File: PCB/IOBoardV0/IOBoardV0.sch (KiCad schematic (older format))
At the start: 28 parts, among them J2 RJ45_2, J3 RJ45_2, J4 RJ45_2, J5 RJ45_2, J6 RJ45_2, J7 RJ45_2, J8 RJ45_2, J9 RJ45_2, P1 RASPBERRY_HAT, U1 74LS04, U2 74LS138, U3 74LS164, U4 74LS373, U5 74LS74, U6 74LS165

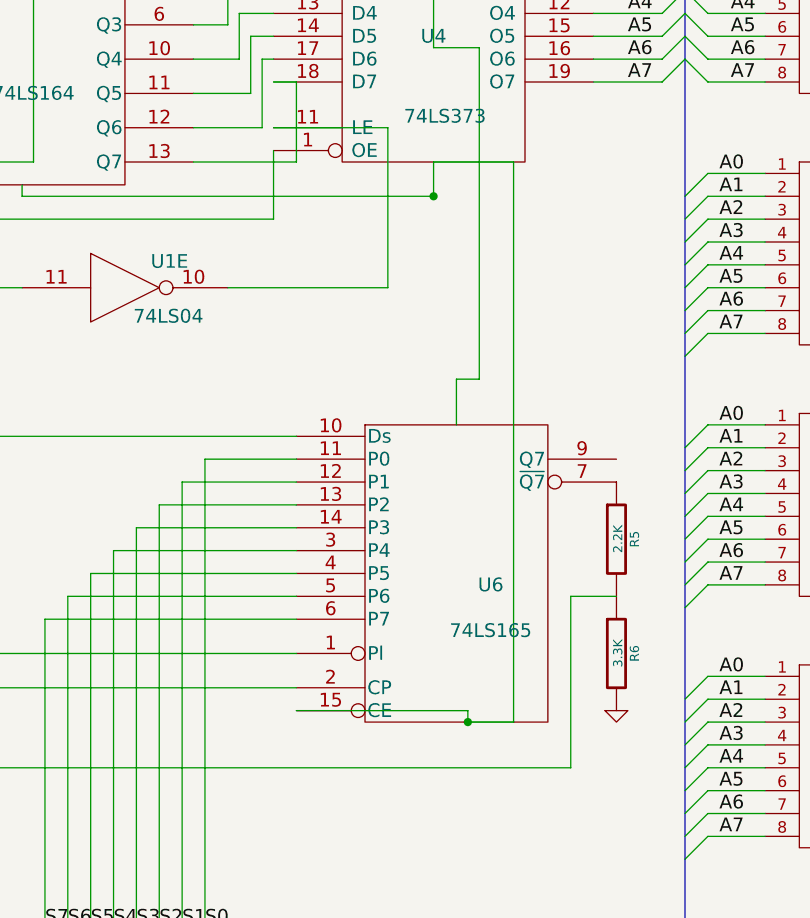
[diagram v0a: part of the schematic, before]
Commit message: Add files via upload
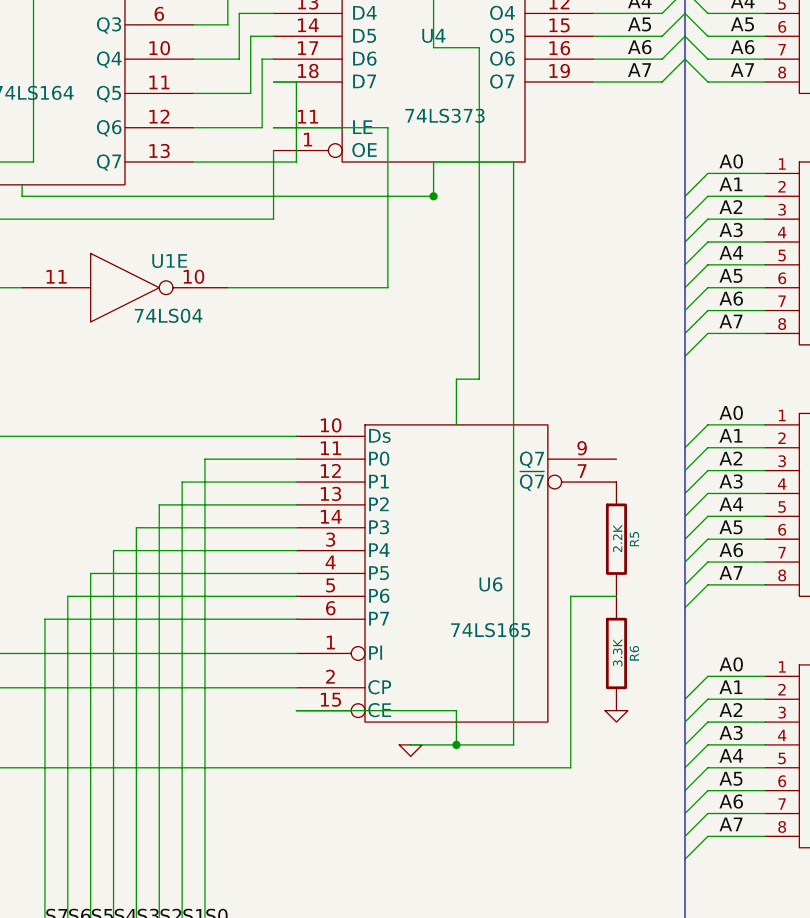
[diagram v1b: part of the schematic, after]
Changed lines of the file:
@@
 Sheet 1 1
 Title ""
-Date "23 apr 2020"
+Date "20 jun 2020"
 Rev ""
 Comp ""
@@
 	5600 4350 7600 4350
 Wire Wire Line
-	7600 4450 8350 4450
-Wire Wire Line
-	8350 4450 8350 4500
-Wire Wire Line
 	8200 2050 8550 2050
 Wire Wire Line
-	8550 2050 8550 4500
+	8550 2050 8550 4600
 Wire Wire Line
 	8200 950  8200 1550
@@
 Wire Wire Line
 	8300 3000 8300 3200
-Connection ~ 8350 4500
-Wire Wire Line
-	8550 4500 8350 4500
 Wire Wire Line
 	6450 850  6400 850
@@
 Connection ~ 2500 5500
 Connection ~ 2500 5900
+Wire Wire Line
+	8550 4600 8100 4600
+Wire Wire Line
+	8300 4600 8300 4450
+Wire Wire Line
+	8300 4450 7600 4450
+$Comp
+L GND #PWR09
+U 1 1 5EEE2585
+P 8100 4600
+F 0 "#PWR09" H 8100 4600 30  0001 C CNN
+F 1 "GND" H 8100 4530 30  0001 C CNN
+F 2 "" H 8100 4600 60  0000 C CNN
+F 3 "" H 8100 4600 60  0000 C CNN
+	1    8100 4600
+	1    0    0    -1
+$EndComp
+Connection ~ 8300 4600
 $EndSCHEMATC
